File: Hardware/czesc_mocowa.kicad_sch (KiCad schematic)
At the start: 20 parts, among them J1 Screw_Terminal_01x02, J2 Screw_Terminal_01x02, Q1 NMOS, Q2 NMOS, Q3 NMOS, Q4 NMOS, U1 IR2102, U2 IR2102

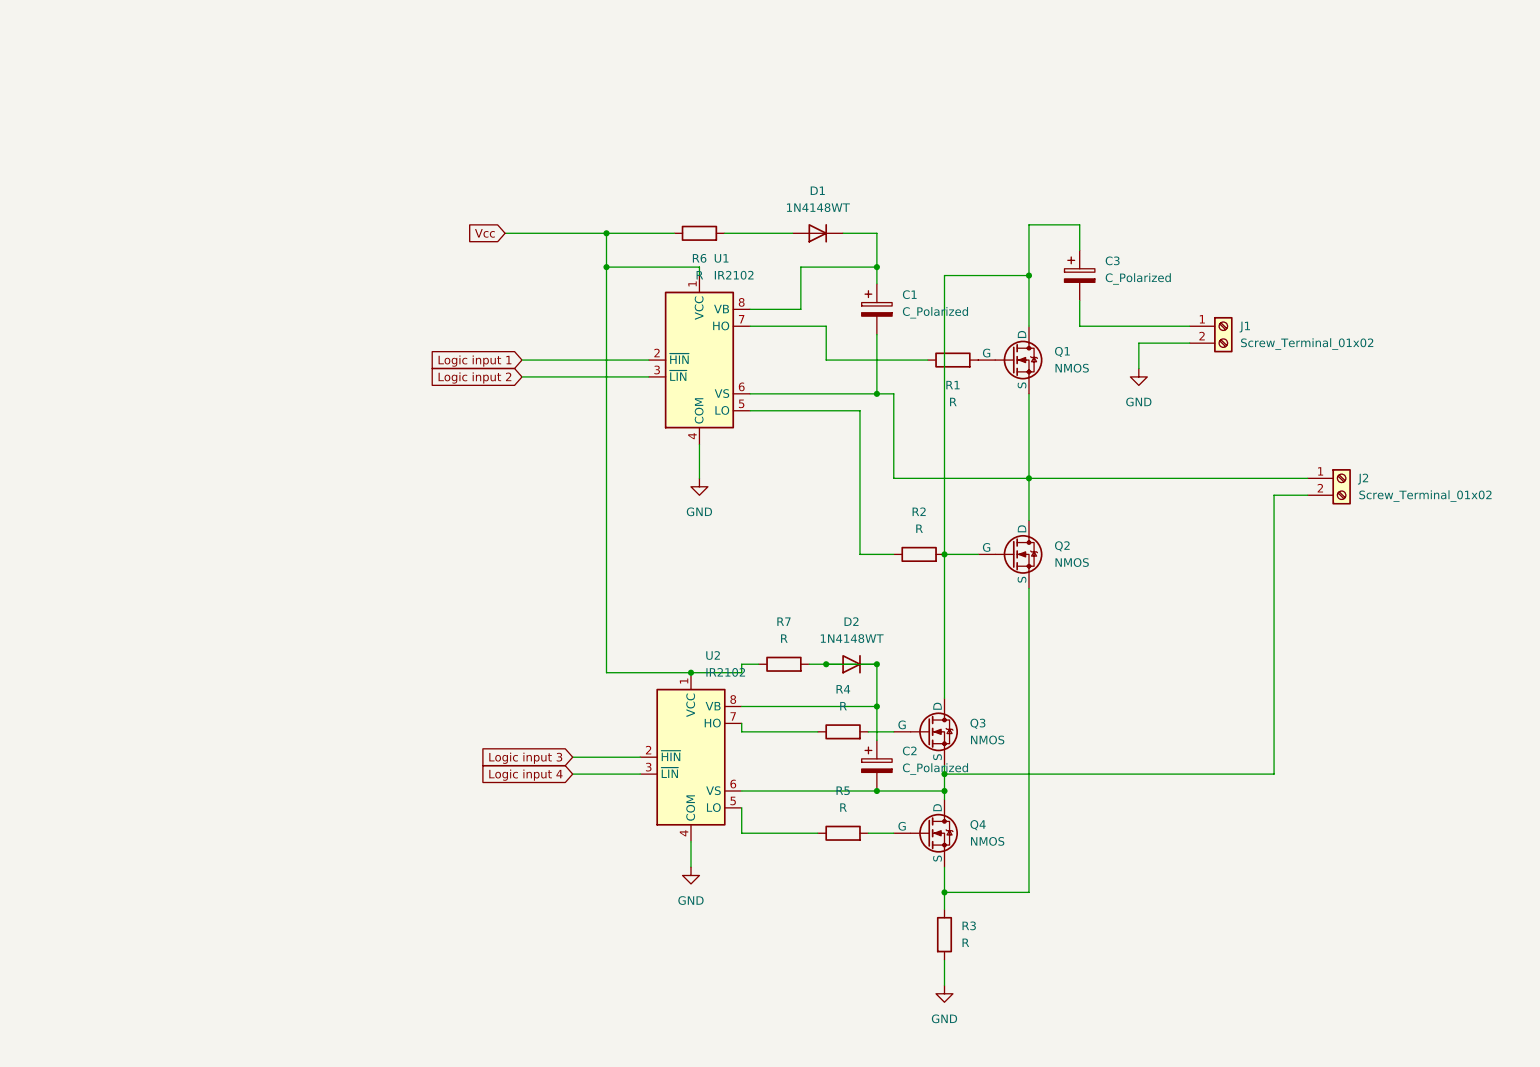
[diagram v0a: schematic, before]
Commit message: Schemat-update
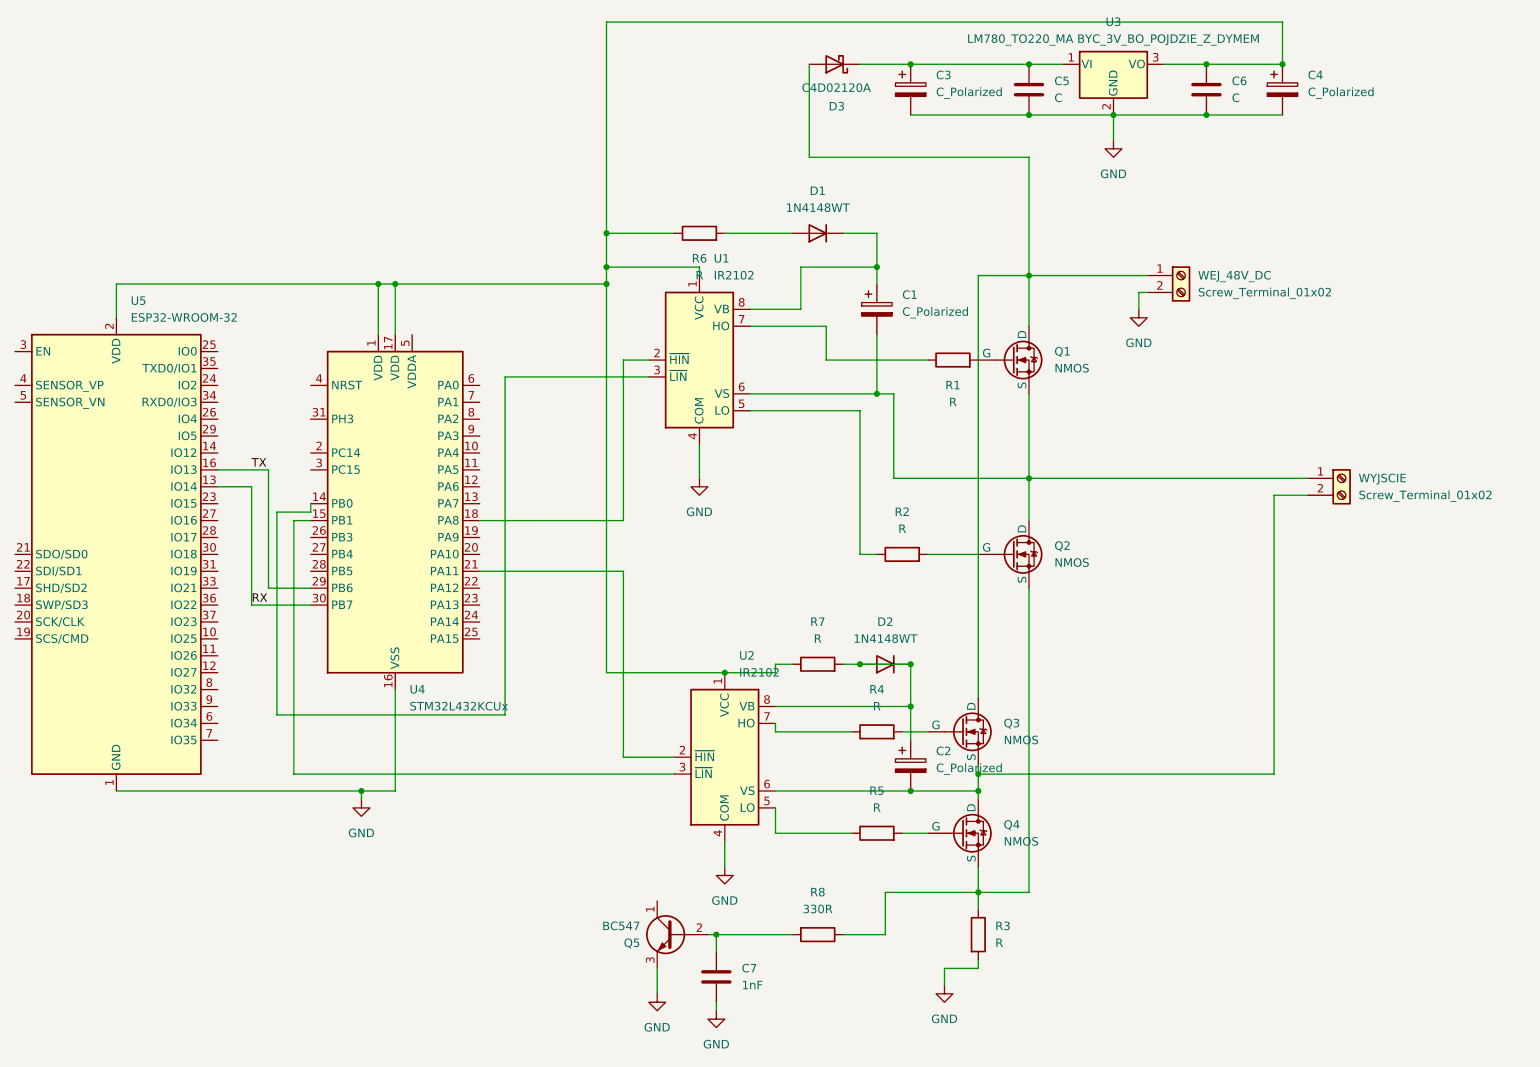
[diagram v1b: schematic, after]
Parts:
- added C4: C_Polarized, symbol Device:C_Polarized
- added C5, C6: C, symbol Device:C
- added C7: 1nF, symbol Device:C
- added D3: C4D02120A, Package_TO_SOT_THT:TO-220-2_Vertical, symbol Diode:C4D02120A
- added Q5: BC547, Package_TO_SOT_THT:TO-92_Inline, symbol Transistor_BJT:BC547
- added R8: 330R, symbol Device:R
- added U3: LM780_TO220_MA BYC_3V_BO_POJDZIE_Z_DYMEM, Package_TO_SOT_THT:TO-220-3_Vertical, symbol Regulator_Linear:LM7805_TO220
- added U4: STM32L432KCUx, Package_DFN_QFN:QFN-32-1EP_5x5mm_P0.5mm_EP3.45x3.45mm, symbol MCU_ST_STM32L4:STM32L432KCUx
- added U5: ESP32-WROOM-32, RF_Module:ESP32-WROOM-32, symbol RF_Module:ESP32-WROOM-32
- renumbered J1 to WEJ_48V_DC, J2 to WYJSCIE
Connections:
- net GND: now also C3.2, C4.2, C5.2, C6.2, C7.1, Q5.3 (E), U3.2 (GND), U4.16 (VSS), U4.32 (VSS), U4.33 (VSS), U5.1 (GND), U5.15 (GND), U5.38 (GND), U5.39 (GND)
- net at WEJ_48V_DC.1 (Pin_1): now also Q1.1 (D), Q3.1 (D), D3.2 (A); no longer C3.2
- net at Q2.3 (S), Q4.3 (S), R3.1: now also R8.1
- net Logic input 1: no longer names the net of U1.2 (~{HIN})
- net Logic input 1: now also U4.18 (PA8)
- net Logic input 2: no longer names the net of U1.3 (~{LIN})
- net Logic input 2: now also U4.14 (PB0)
- net Logic input 3: no longer names the net of U2.2 (~{HIN})
- net Logic input 3: now also U4.21 (PA11)
- net Logic input 4: no longer names the net of U2.3 (~{LIN})
- net Logic input 4: now also U4.15 (PB1)
- net Vcc: no longer names the net of R6.1, R7.1, U1.1 (VCC), U2.1 (VCC)
- net Vcc: now also C4.1, C6.1, U3.3 (VO), U4.1 (VDD), U4.17 (VDD), U5.2 (VDD)
- new net: C7.2, Q5.2 (B), R8.2
- new net: Q2.2 (G), R2.2
- new net: C3.1, C5.1, D3.1 (K), U3.1 (VI)
- new net RX: U4.30 (PB7), U5.13 (IO14)
- new net TX: U4.29 (PB6), U5.16 (IO13)
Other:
- moved on the sheet: C2, D2, Q3, Q4, R2, R3, R4, R5, R7, U2, WEJ_48V_DC
